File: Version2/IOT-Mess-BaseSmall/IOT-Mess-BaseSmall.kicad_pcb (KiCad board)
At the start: 2 copper layers, 98.5 x 32.8 mm, 6 parts, among them J1 ESP_P16 / ESP12, J2 ESP_P16 / C3, J22 Lolin32, J3 ESP_P40, J6 CH582

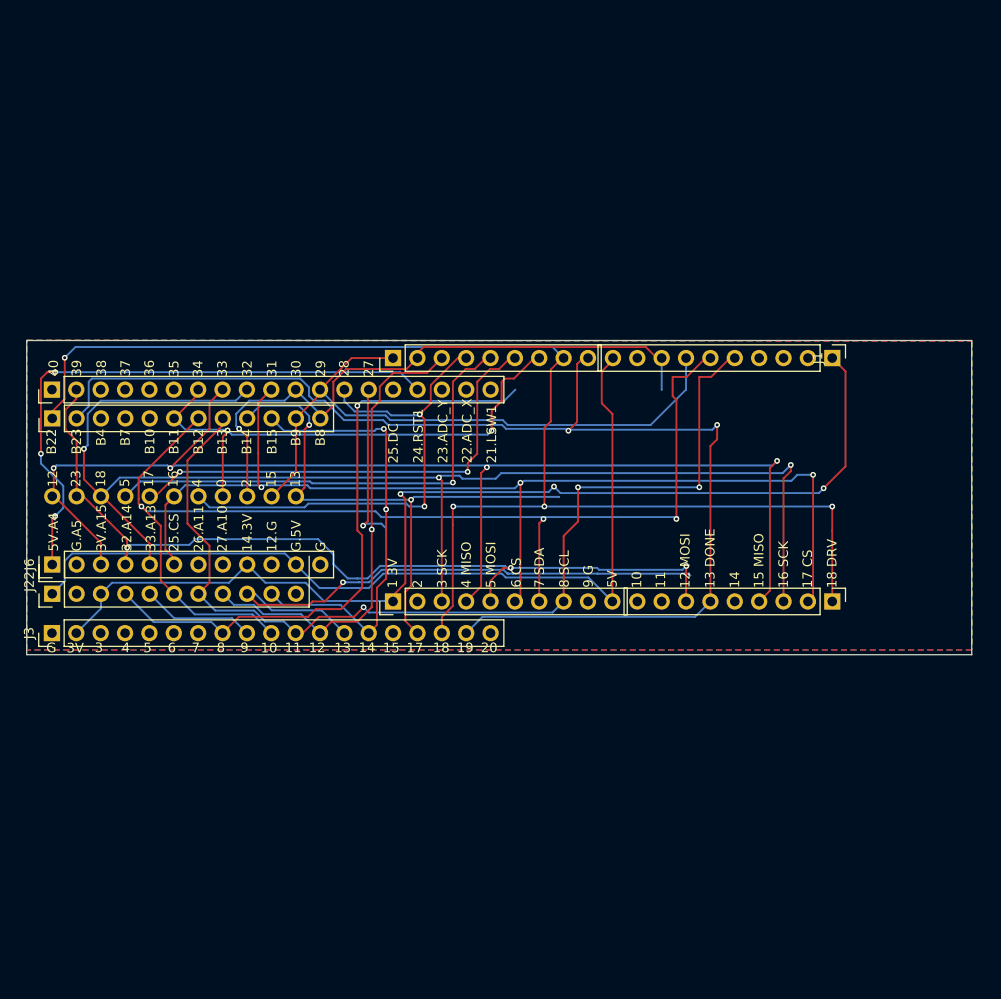
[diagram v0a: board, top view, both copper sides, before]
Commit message: added jumper boards.
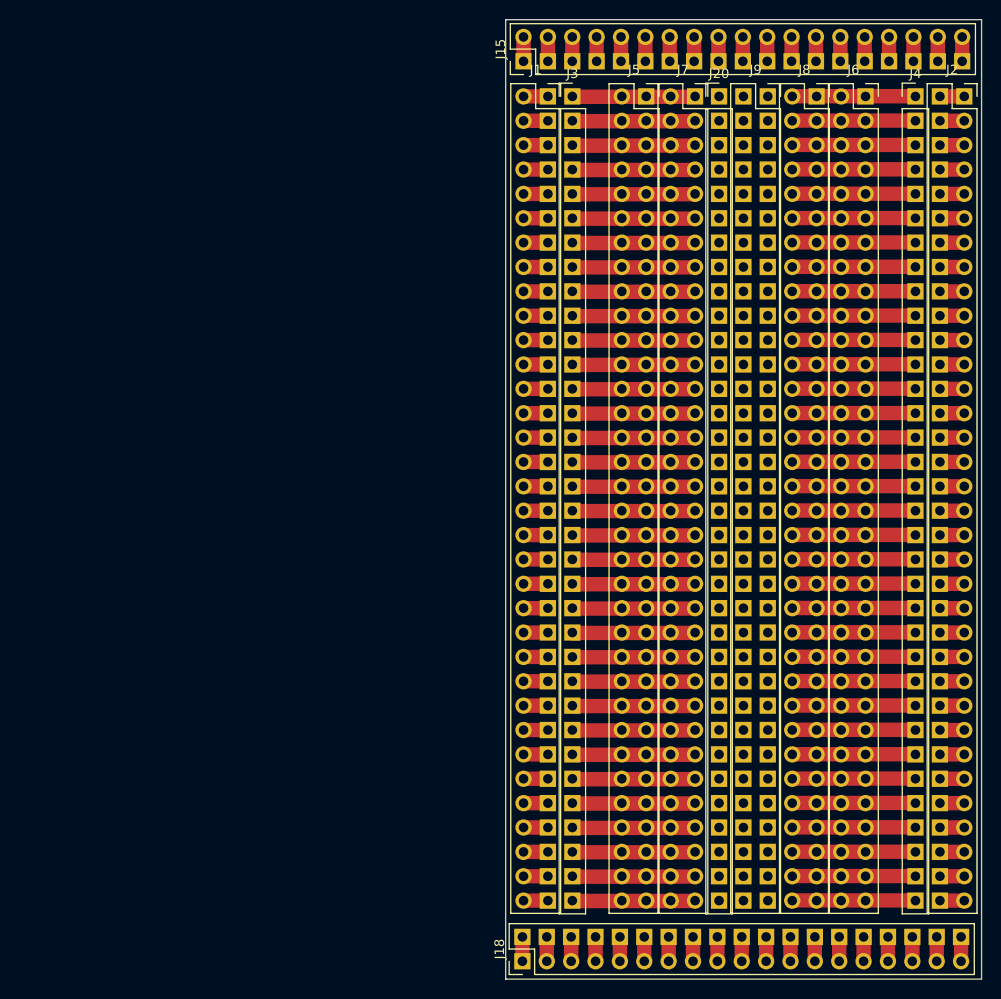
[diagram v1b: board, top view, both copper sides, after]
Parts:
- removed G***: LOGO, IOT-Mess-Footprints:catIcon8x8
- removed J22: Lolin32, IOT-Mess-Footprints:Lolin32-Adapter
- added J15: Conn_02x19_Odd_Even, Connector_PinHeader_2.54mm:PinHeader_2x19_P2.54mm_Vertical, F.Cu at (121.3, 56.6)
- added J18: Conn_02x19_Odd_Even, Connector_PinHeader_2.54mm:PinHeader_2x19_P2.54mm_Vertical, F.Cu at (121.2, 150.4)
- added J20: Conn_01x34_Pin, Connector_PinHeader_2.54mm:PinHeader_1x34_P2.54mm_Vertical, F.Cu at (141.7, 60.3)
- added J4: Conn_01x34_Pin, Connector_PinHeader_2.54mm:PinHeader_1x34_P2.54mm_Vertical, F.Cu at (162.2, 60.3)
- added J5: Conn_02x34_Odd_Even, Connector_PinSocket_2.54mm:PinSocket_2x34_P2.54mm_Vertical, F.Cu at (134.1, 60.3)
- added J7: Conn_02x34_Odd_Even, Connector_PinSocket_2.54mm:PinSocket_2x34_P2.54mm_Vertical, F.Cu at (139.2, 60.3)
- added J8: Conn_02x34_Odd_Even, Connector_PinSocket_2.54mm:PinSocket_2x34_P2.54mm_Vertical, F.Cu at (151.9, 60.3)
- added J9: Conn_02x34_Odd_Even, Connector_PinSocket_2.54mm:PinSocket_2x34_P2.54mm_Vertical, F.Cu at (146.8, 60.3)
- J1: value ESP_P16 / ESP12 -> Conn_02x34_Odd_Even; footprint IOT-Mess-Footprints:ESP_P16 -> Connector_PinSocket_2.54mm:PinSocket_2x34_P2.54mm_Vertical
- J2: value ESP_P16 / C3 -> Conn_02x34_Odd_Even; footprint IOT-Mess-Footprints:ESP_P16 -> Connector_PinSocket_2.54mm:PinSocket_2x34_P2.54mm_Vertical
- J3: value ESP_P40 -> Conn_01x34_Pin; footprint IOT-Mess-Footprints:ESP_P40 -> Connector_PinHeader_2.54mm:PinHeader_1x34_P2.54mm_Vertical
- J6: value CH582 -> Conn_02x34_Odd_Even; footprint IOT-Mess-Footprints:CH582_Base -> Connector_PinSocket_2.54mm:PinSocket_2x34_P2.54mm_Vertical
- moved J6 97.8 mm to (157.0, 60.3), turned to 0 degrees
- moved J2 79.5 mm to (167.3, 60.3), turned to 0 degrees
- moved J3 77.9 mm to (126.4, 60.3), turned to 0 degrees
- moved J1 40.3 mm to (123.9, 60.3), turned to 0 degrees
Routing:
- net DRIVE: track 139.0 -> 0.00 mm, vias 4 -> 0
- net SCK: track 137.8 -> 0.00 mm, vias 3 -> 0
- net MISO: track 129.4 -> 0.00 mm, vias 4 -> 0
- net DONE: track 126.7 -> 0.00 mm, vias 2 -> 0
- net SDA: track 119.0 -> 0.00 mm, vias 3 -> 0
- net CS: track 113.0 -> 0.00 mm, vias 3 -> 0
- net +3.3V: track 110.0 -> 0.00 mm, vias 3 -> 0
- net SCL: track 103.5 -> 0.00 mm, vias 3 -> 0
- net MOSI: track 92.3 -> 0.00 mm, vias 3 -> 0
- net 5V: track 90.8 -> 0.00 mm
- net DC: track 66.2 -> 0.00 mm
- net SDA2: track 64.7 -> 0.00 mm, vias 1 -> 0
- net RST1: track 64.3 -> 0.00 mm, vias 1 -> 0
- net CS_1: track 61.1 -> 0.00 mm, vias 3 -> 0
- net SCK2: track 60.3 -> 0.00 mm, vias 1 -> 0
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- removed copper zone on B.Cu, net GND
- removed copper zone on F.Cu, net GND
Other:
- board size 98.5 x 32.8 mm -> 49.6 x 100 mm
- board text removed: "0"
- board text removed: "1 3V"
- board text removed: "10"
- board text removed: "11"
- board text removed: "12"
- board text removed: "12 MOSI"
- board text removed: "12.G"
- board text removed: "13"
- board text removed: "13 DONE"
- board text removed: "14"
- board text removed: "14.3V"
- board text removed: "15"
- board text removed: "15 MISO"
- board text removed: "16"
- board text removed: "16 SCK"
- board text removed: "17"
- board text removed: "17 CS"
- board text removed: "18"
- board text removed: "18 DRV"
- board text removed: "19"
- board text removed: "2"
- board text removed: "20"
- board text removed: "21.LSW1"
- board text removed: "22.ADC_X"
- board text removed: "23"
- board text removed: "23.ADC_Y"
- board text removed: "24.RST1"
- board text removed: "25.CS"
- board text removed: "25.DC"
- board text removed: "26.A11"
- board text removed: "27"
- board text removed: "27.A10"
- board text removed: "28"
- board text removed: "29"
- board text removed: "3"
- board text removed: "3 SCK"
- board text removed: "30"
- board text removed: "31"
- board text removed: "32"
- board text removed: "32.A14"
- board text removed: "33"
- board text removed: "33.A13"
- board text removed: "34"
- board text removed: "35"
- board text removed: "36"
- board text removed: "37"
- board text removed: "38"
- board text removed: "39"
- board text removed: "3V"
- board text removed: "3V.A15"
- board text removed: "4"
- board text removed: "4 MISO"
- board text removed: "40"
- board text removed: "5"
- board text removed: "5 MOSI"
- board text removed: "5V"
- board text removed: "5V.A4"
- board text removed: "6"
- board text removed: "6 CS"
- board text removed: "7"
- board text removed: "7 SDA"
- board text removed: "8"
- board text removed: "8 SCL"
- board text removed: "9"
- board text removed: "9 G"
- board text removed: "B10"
- board text removed: "B11"
- board text removed: "B12"
- board text removed: "B13"
- board text removed: "B14"
- board text removed: "B15"
- board text removed: "B22"
- board text removed: "B23"
- board text removed: "B4"
- board text removed: "B7"
- board text removed: "B8"
- board text removed: "B9"
- board text removed: "G"
- board text removed: "G.5V"
- board text removed: "G.A5"
- board text removed: "IOT_Mess AdapterB V1.0 07/05/25"
